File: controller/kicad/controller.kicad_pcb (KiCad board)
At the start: 2 copper layers, 132.3 x 80.9 mm, 6 parts, among them J1 pcie_98, J2 pcie_98, J3 pcie_98, J4 pcie_98, J5 pcie_98

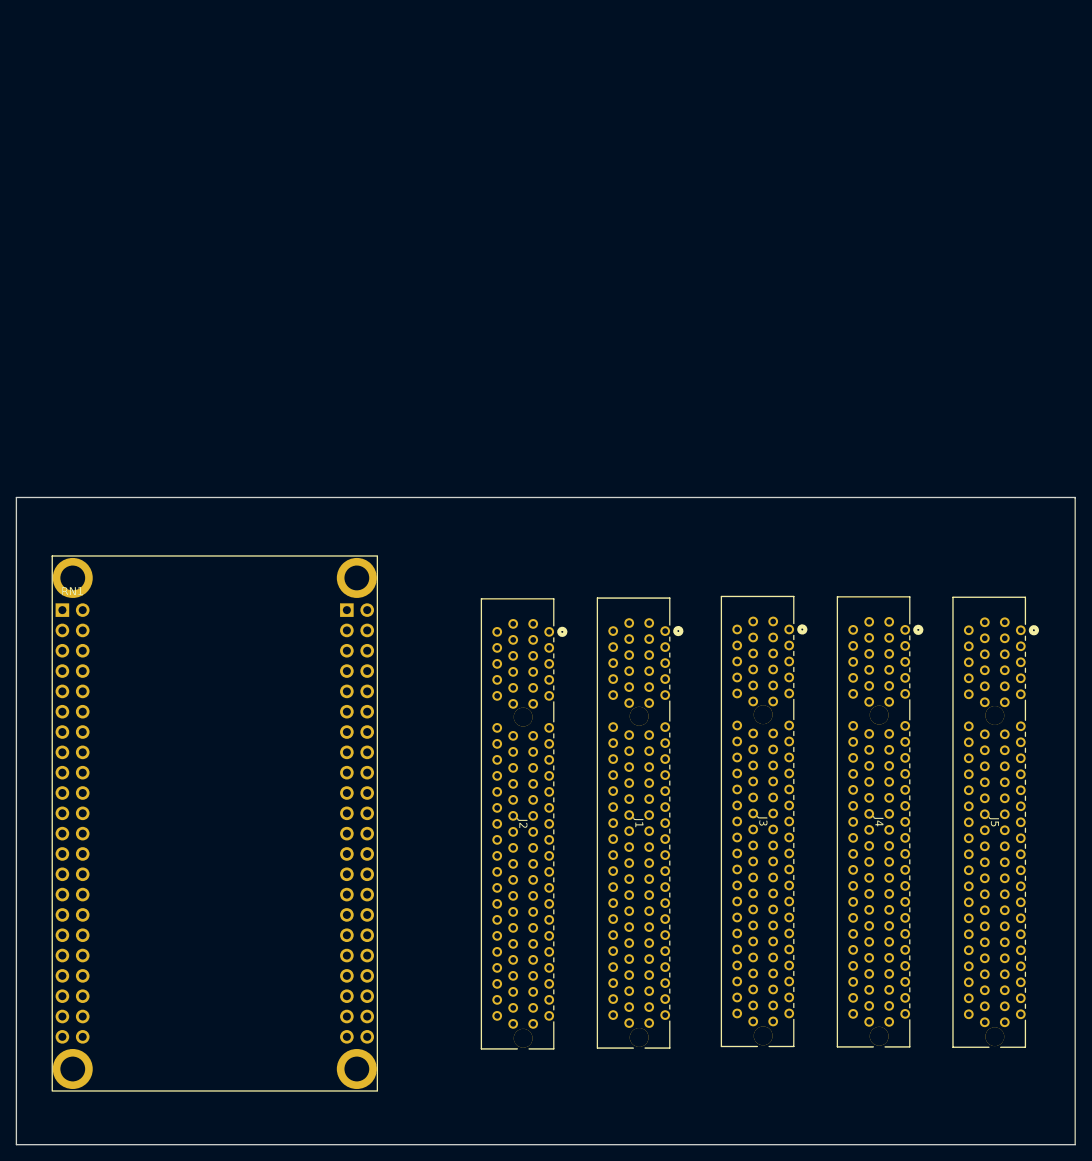
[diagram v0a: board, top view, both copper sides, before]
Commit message: Work in progress. Controller schematic.
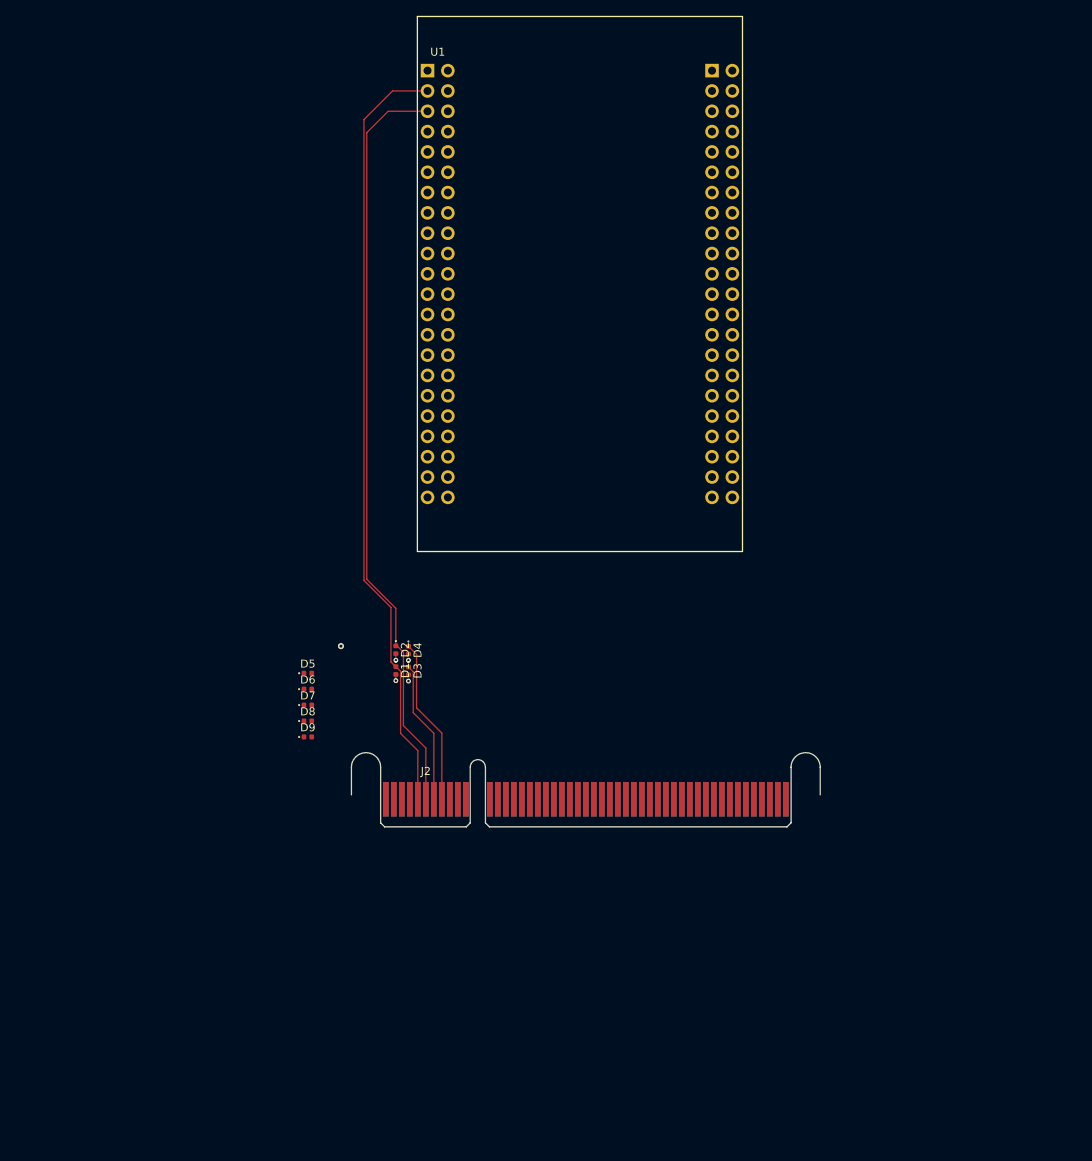
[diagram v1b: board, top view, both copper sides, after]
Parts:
- removed J1, J3, J4, J5: pcie_98, controller:pcie_98_socket
- removed RN1: R_Pack06, controller:weact_stm32fh750
- added D1: ESD, Diode_SMD:D_0402_1005Metric, F.Cu at (62.2, 42.9)
- added D2: ESD, Diode_SMD:D_0402_1005Metric, F.Cu at (62.2, 40.3)
- added D3: ESD, Diode_SMD:D_0402_1005Metric, F.Cu at (63.8, 43.0)
- added D4: ESD, Diode_SMD:D_0402_1005Metric, F.Cu at (63.8, 40.4)
- added D5: ESD, Diode_SMD:D_0402_1005Metric, F.Cu at (51.2, 43.3)
- added D6: ESD, Diode_SMD:D_0402_1005Metric, F.Cu at (51.2, 45.3)
- added D7: ESD, Diode_SMD:D_0402_1005Metric, F.Cu at (51.2, 47.3)
- added D8: ESD, Diode_SMD:D_0402_1005Metric, F.Cu at (51.2, 49.2)
- added D9: ESD, Diode_SMD:D_0402_1005Metric, F.Cu at (51.2, 51.2)
- added U1: WeAct_STM32H750_Module, controller:weact_stm32fh750, F.Cu at (85.2, -5.38)
- J2: footprint controller:pcie_98_socket -> controller:pcie_98_edge
- moved J2 26.3 mm to (72.5, 62.5), turned to 0 degrees
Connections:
- J2 pad A1: (no net) -> GND
- J2 pad A10: (no net) -> /A
- J2 pad A11: (no net) -> /A
- J2 pad A12: (no net) -> /A
- J2 pad A13: (no net) -> /A
- J2 pad A14: (no net) -> /A
- J2 pad A15: (no net) -> /A
- J2 pad A16: (no net) -> /A
- J2 pad A17: (no net) -> /A
- J2 pad A18: (no net) -> /A
- J2 pad A19: (no net) -> /A
- J2 pad A2: (no net) -> GND
- J2 pad A20: (no net) -> /A
- J2 pad A21: (no net) -> /A
- J2 pad A22: (no net) -> /A
- J2 pad A23: (no net) -> /A
- J2 pad A24: (no net) -> /A
- J2 pad A25: (no net) -> /A
- J2 pad A26: (no net) -> /A
- J2 pad A27: (no net) -> /A
- J2 pad A28: (no net) -> /A
- J2 pad A29: (no net) -> /A
- J2 pad A3: (no net) -> GND
- J2 pad A30: (no net) -> /A
- J2 pad A31: (no net) -> /A
- J2 pad A32: (no net) -> /A
- J2 pad A33: (no net) -> /A
- J2 pad A34: (no net) -> /A
- J2 pad A35: (no net) -> /A
- J2 pad A36: (no net) -> /A
- J2 pad A37: (no net) -> /A
- J2 pad A38: (no net) -> /A
- J2 pad A39: (no net) -> /A
- J2 pad A4: (no net) -> GND
- J2 pad A40: (no net) -> /A
- J2 pad A41: (no net) -> /A
- J2 pad A42: (no net) -> /A
- J2 pad A43: (no net) -> /A
- J2 pad A44: (no net) -> /A
- J2 pad A45: (no net) -> /A
- J2 pad A46: (no net) -> /A
- J2 pad A47: (no net) -> /A
- J2 pad A48: (no net) -> /VIN-
- J2 pad A49: (no net) -> /VIN-
- J2 pad A5: (no net) -> /PE0
- J2 pad A6: (no net) -> /PB8
- J2 pad A7: (no net) -> /PB6
- J2 pad A8: (no net) -> /PB4
- J2 pad A9: (no net) -> /PD7
- J2 pad B1: (no net) -> +5V
- J2 pad B10: (no net) -> /B
- J2 pad B11: (no net) -> /B
- J2 pad B12: (no net) -> /B
- J2 pad B13: (no net) -> /B
- J2 pad B14: (no net) -> /B
- J2 pad B15: (no net) -> /B
- J2 pad B16: (no net) -> /B
- J2 pad B17: (no net) -> /B
- J2 pad B18: (no net) -> /B
- J2 pad B19: (no net) -> /B
- J2 pad B2: (no net) -> +5V
- J2 pad B20: (no net) -> /B
- J2 pad B21: (no net) -> /B
- J2 pad B22: (no net) -> /B
- J2 pad B23: (no net) -> /B
- J2 pad B3: (no net) -> +5V
- J2 pad B4: (no net) -> +5V
- J2 pad B5: (no net) -> /PE1
- J2 pad B6: (no net) -> /PB9
- J2 pad B7: (no net) -> /PB7
- J2 pad B8: (no net) -> /PB5
- J2 pad B9: (no net) -> /PB3
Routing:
- net /PE1: track 0.00 -> 97.2 mm
- net /PB9: track 0.00 -> 95.1 mm
- net /PB5: track 0.00 -> 20.9 mm
- net /PB7: track 0.00 -> 17.8 mm
- net GND: track 0.00 -> 1.77 mm, vias 0 -> 4
- net (no net): vias 0 -> 1
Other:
- board size 132.3 x 80.9 mm -> 58.6 x 9.3 mm
